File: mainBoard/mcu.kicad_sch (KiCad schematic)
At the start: 25 parts, among them SW2 SW_SPDT, SW3 SW_Push, SW4 SW_Push, U4 STM32F401RETx, Y1 ATS240C-E

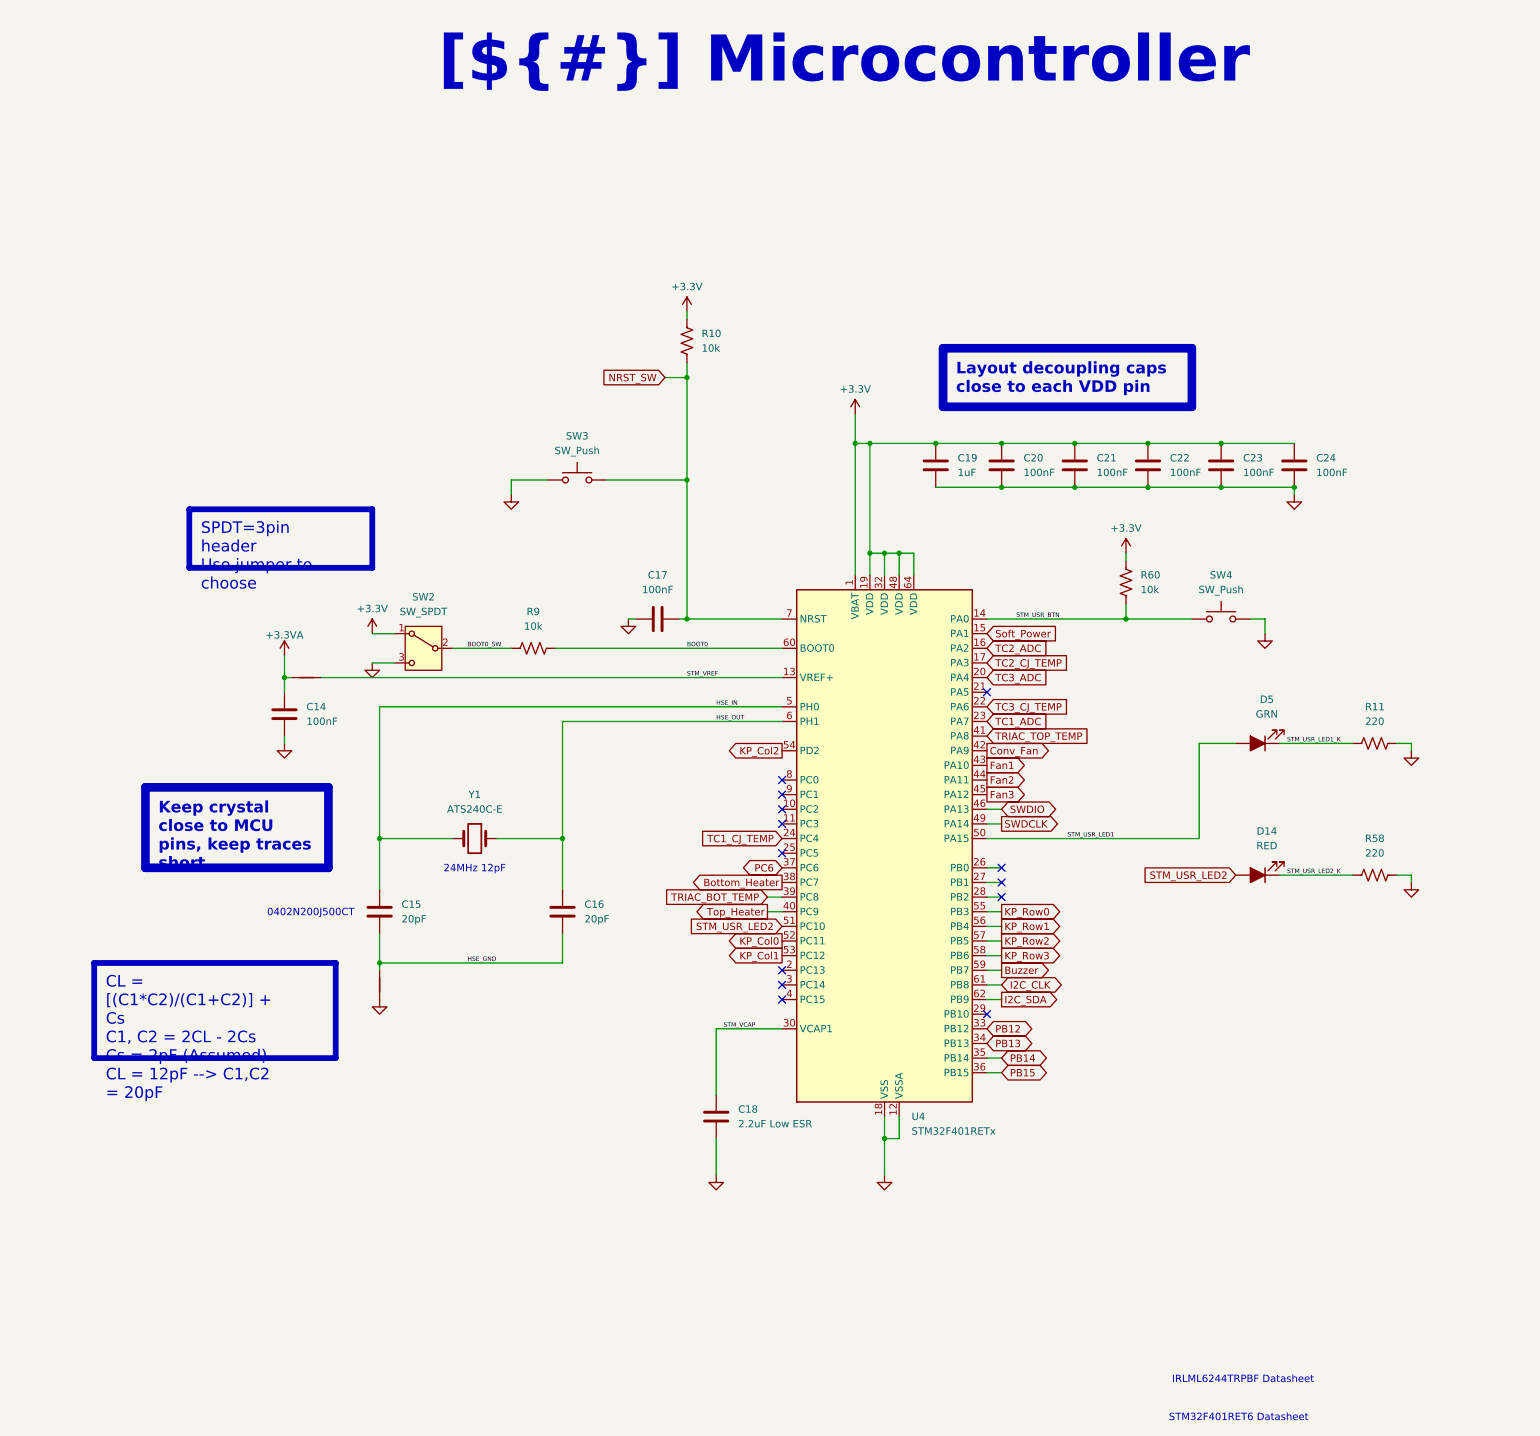
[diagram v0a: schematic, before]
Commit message: Nearly finished with board after revisions
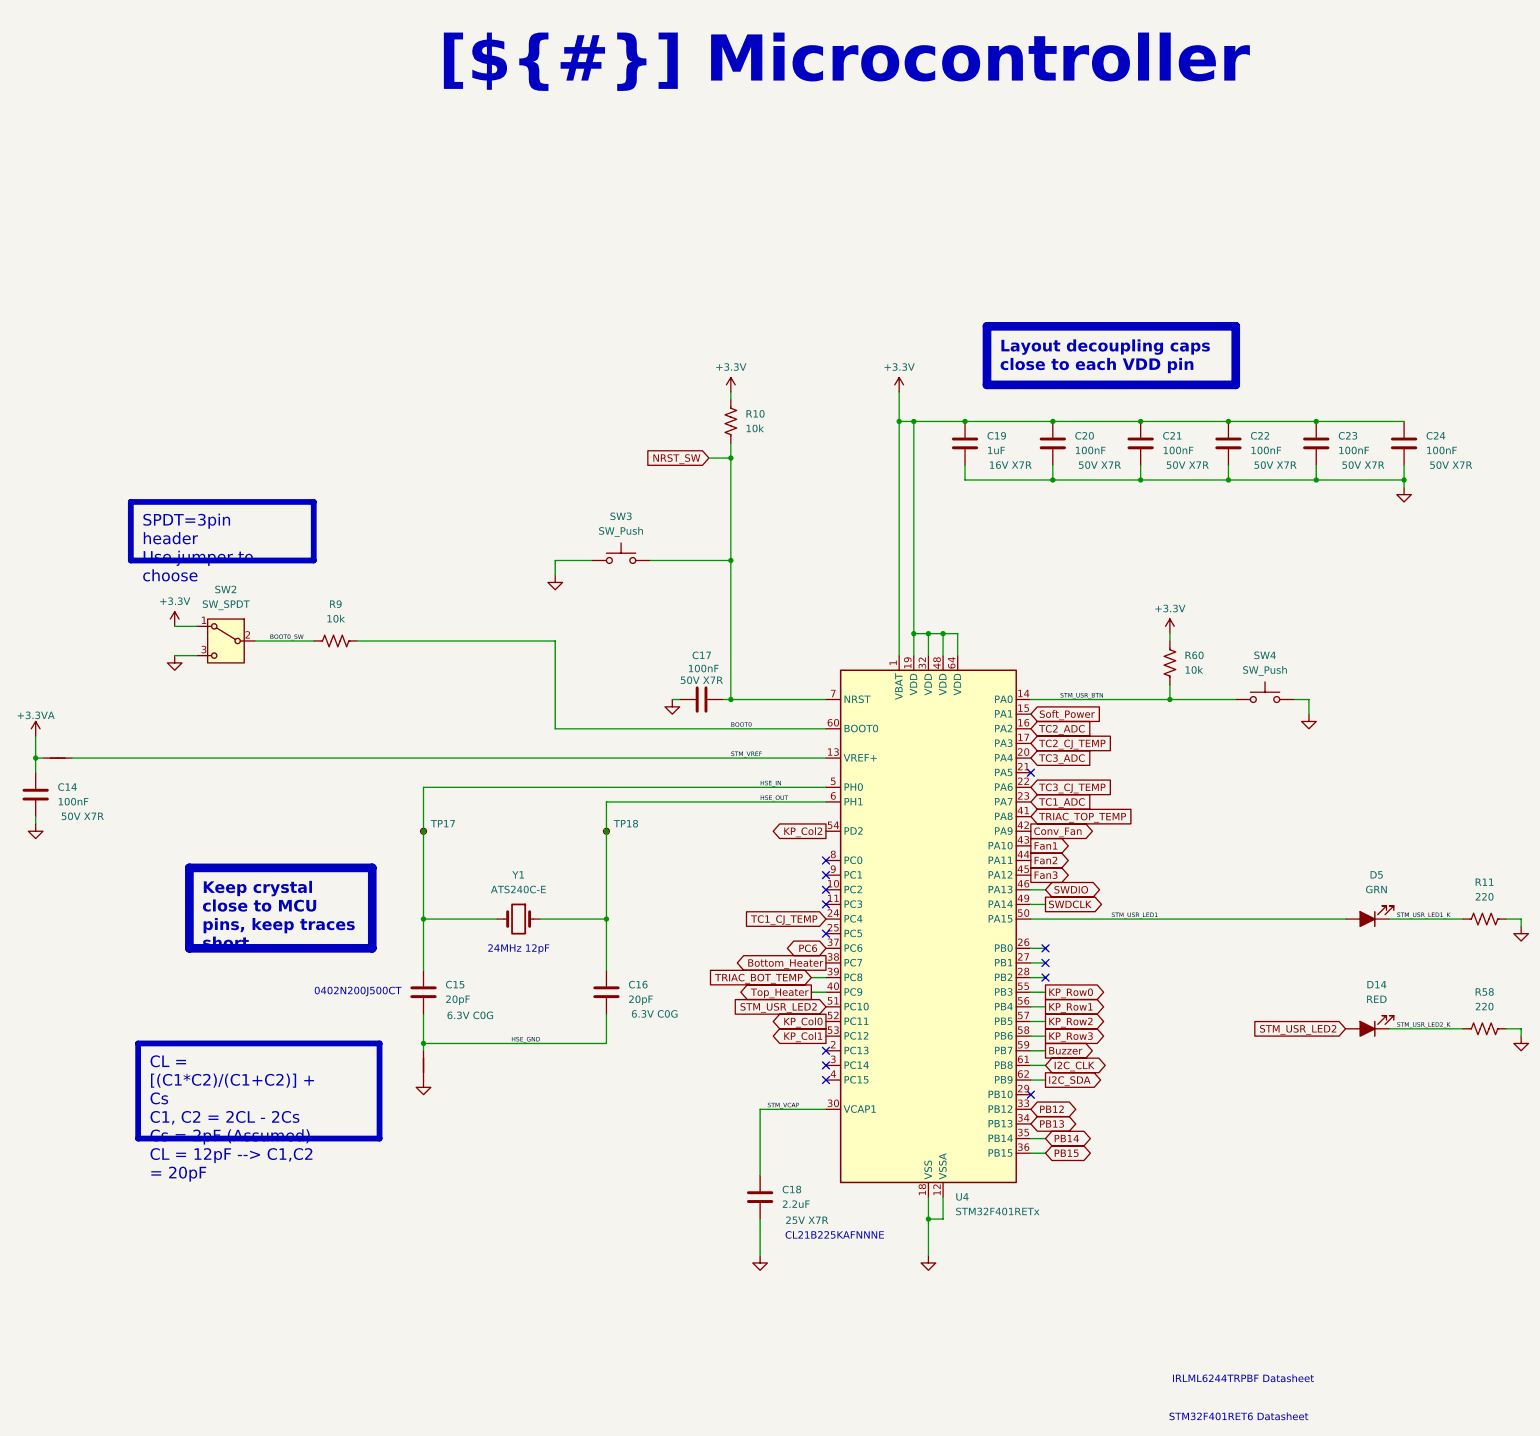
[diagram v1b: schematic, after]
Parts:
- added TP17, TP18: TestPoint_Small, TestPoint:TestPoint_Pad_D1.0mm, symbol Connector:TestPoint_Small
- C14, C17, C20, C21, C22, C23, C24: Type (none) -> 50V X7R
- C15, C16: Type (none) -> 6.3V C0G; part number (none) -> 0402N200J500CT
- C18: value 2.2uF Low ESR -> 2.2uF; Type (none) -> 25V X7R; part number (none) -> CL21B225KAFNNNE
- C19: Type (none) -> 16V X7R
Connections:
- net HSE_IN: now also TP17.1
- net HSE_OUT: now also TP18.1
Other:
- note added: "CL21B225KAFNNNE"
- moved on the sheet: C15, C16, C18, C19, D14, D5, R10, R11, R58, R60, R9, SW2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
